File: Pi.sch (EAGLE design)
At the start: 9 parts, among them X1 RASPI_GPIO_B+#_BOX, X2 HDD, 5V 700mA

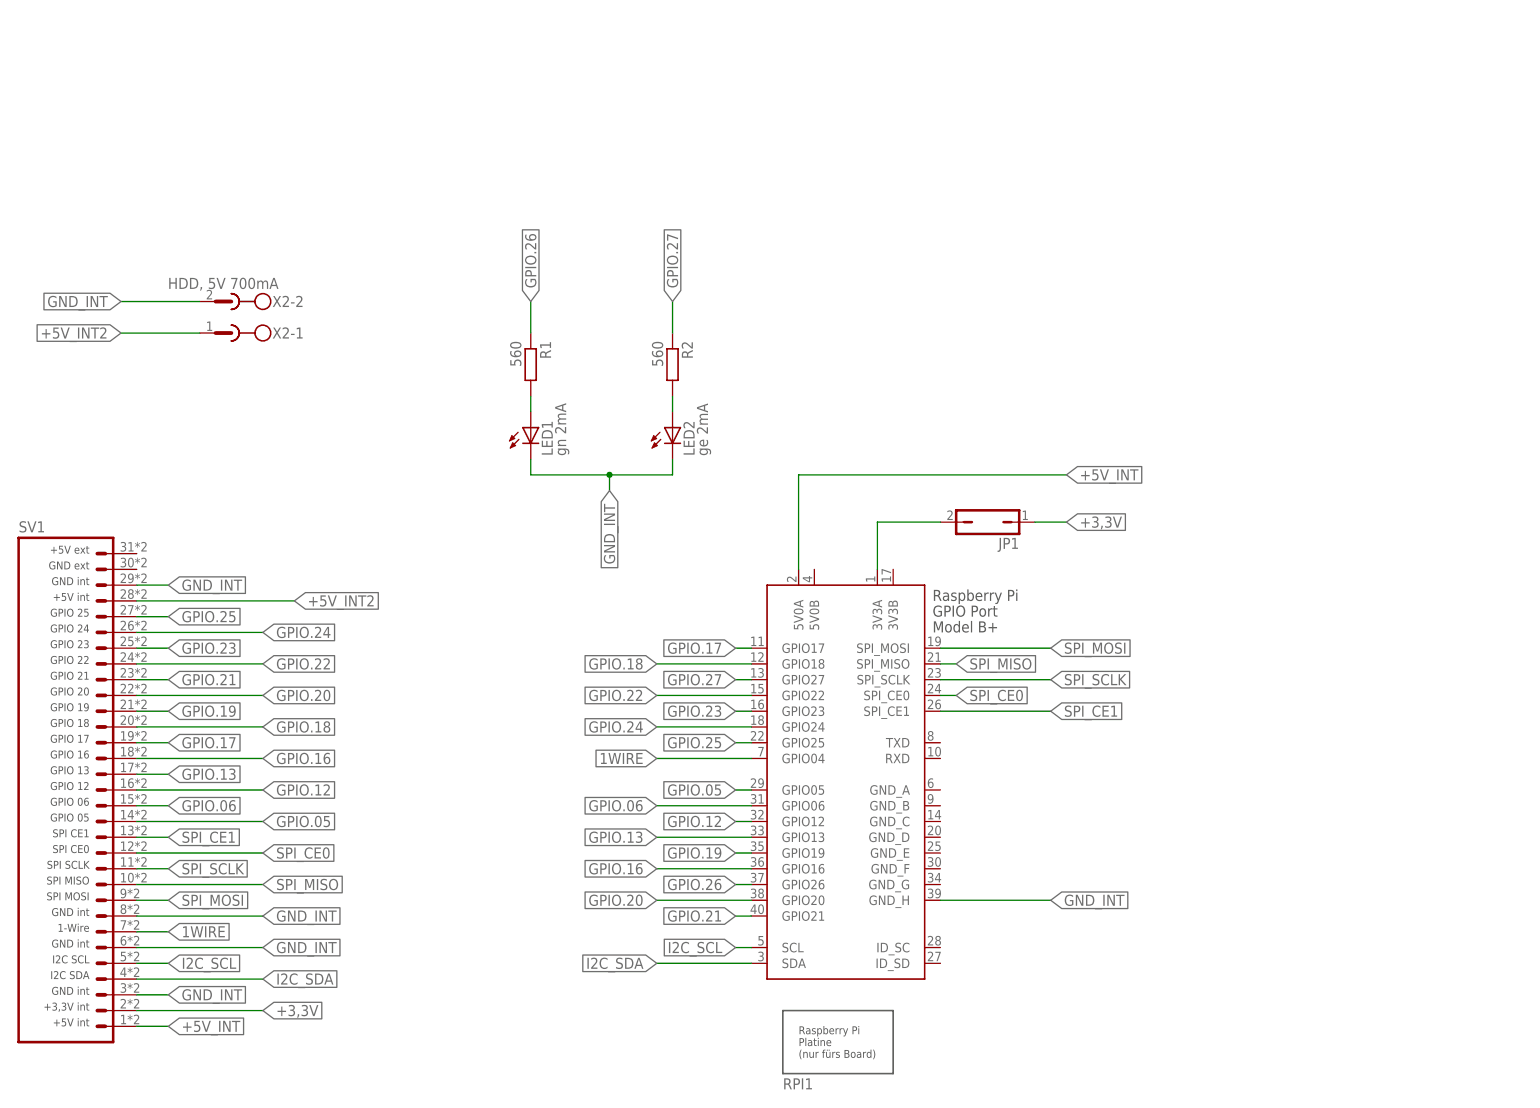
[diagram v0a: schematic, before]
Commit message: Pi und Stromversorgung Rev. 2019
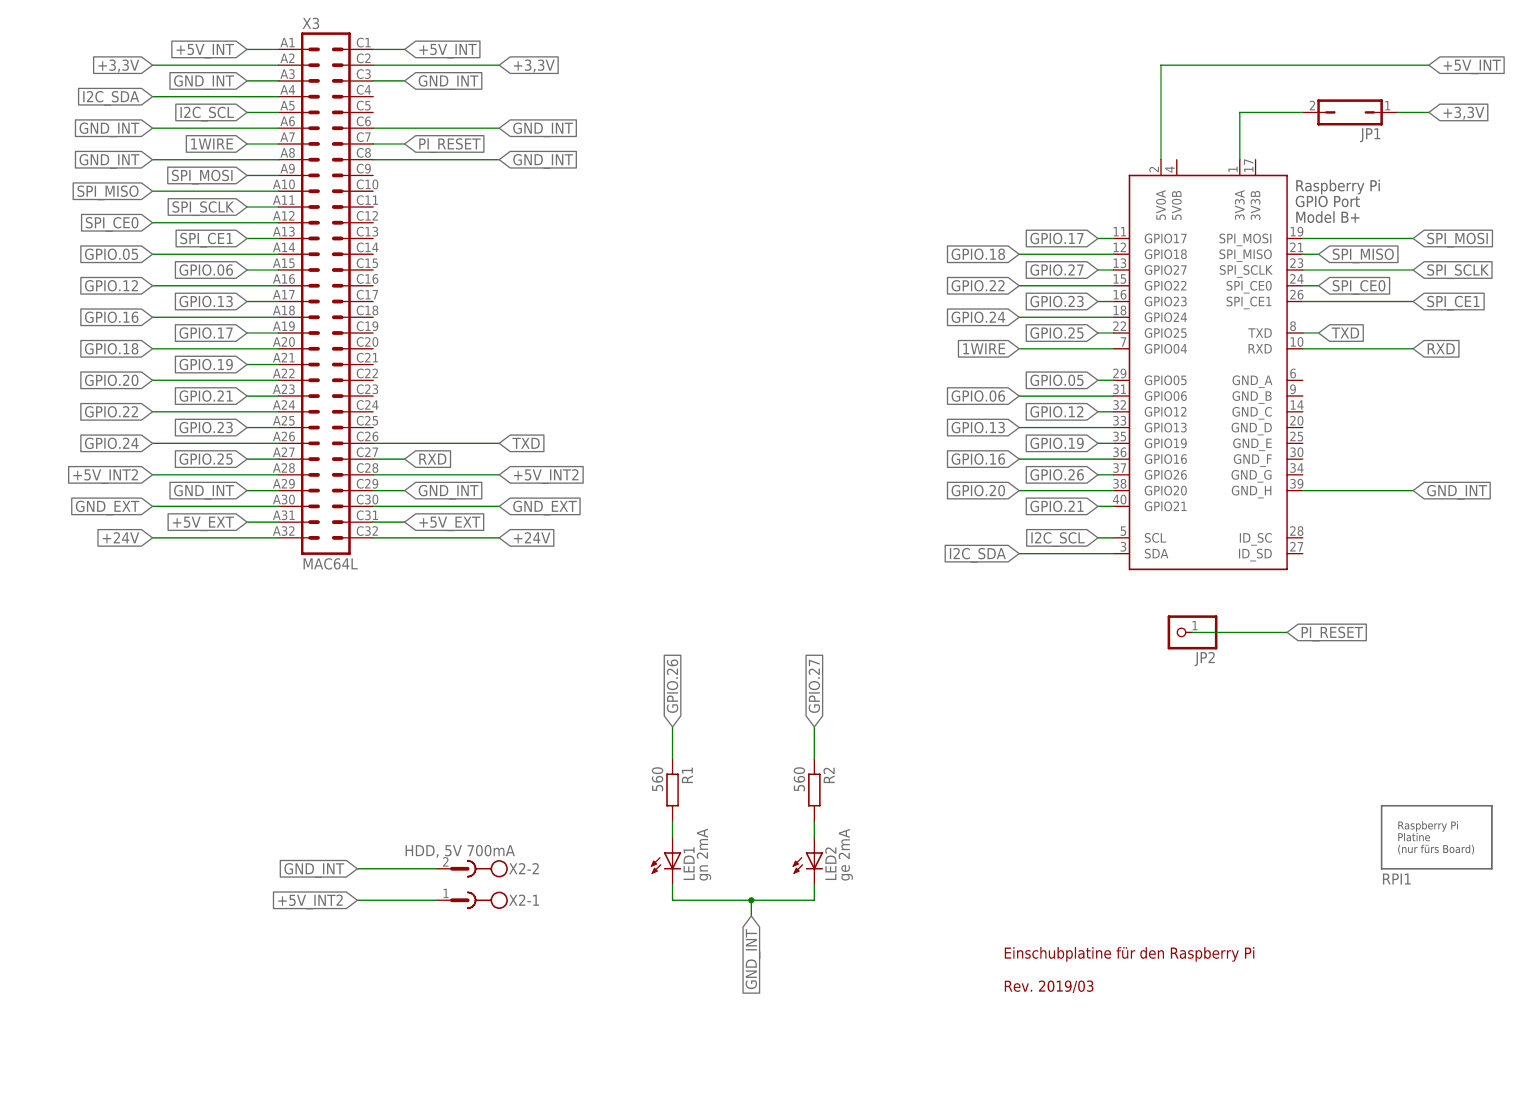
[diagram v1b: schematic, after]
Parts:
- removed SV1: PLATINENVERBINDER-31SMD, homepi:PLATINENVERBINDER-31SMD
- added JP2: (no value), pinhead:PINHD-1X1
- added X3: MAC64L, con-vg:MAC64L
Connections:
- new net +24V: X3.A32, X3.C32
- new net +5V_EXT: X3.A31, X3.C31
- new net GND_EXT: X3.A30, X3.C30
- new net PI_RESET: JP2.1, X3.C7
- new net RXD: X1.RXD, X3.C27
- new net TXD: X1.TXD, X3.C26
- net +3,3V: now also X3.A2, X3.C2; no longer SV1.2
- net +5V_INT: now also X3.A1, X3.C1; no longer SV1.1
- net +5V_INT2: now also X3.A28, X3.C28; no longer SV1.28
- net 1WIRE: now also X3.A7; no longer SV1.7
- net GND_INT: now also X3.A29, X3.A3, X3.A6, X3.A8, X3.C29, X3.C3, X3.C6, X3.C8; no longer SV1.29, SV1.3, SV1.6, SV1.8
- net GPIO.05: now also X3.A14; no longer SV1.14
- net GPIO.06: now also X3.A15; no longer SV1.15
- net GPIO.12: now also X3.A16; no longer SV1.16
- net GPIO.13: now also X3.A17; no longer SV1.17
- net GPIO.16: now also X3.A18; no longer SV1.18
- net GPIO.17: now also X3.A19; no longer SV1.19
- net GPIO.18: now also X3.A20; no longer SV1.20
- net GPIO.19: now also X3.A21; no longer SV1.21
- net GPIO.20: now also X3.A22; no longer SV1.22
- net GPIO.21: now also X3.A23; no longer SV1.23
- net GPIO.22: now also X3.A24; no longer SV1.24
- net GPIO.23: now also X3.A25; no longer SV1.25
- net GPIO.24: now also X3.A26; no longer SV1.26
- net GPIO.25: now also X3.A27; no longer SV1.27
- net I2C_SCL: now also X3.A5; no longer SV1.5
- net I2C_SDA: now also X3.A4; no longer SV1.4
- net SPI_CE0: now also X3.A12; no longer SV1.12
- net SPI_CE1: now also X3.A13; no longer SV1.13
- net SPI_MISO: now also X3.A10; no longer SV1.10
- net SPI_MOSI: now also X3.A9; no longer SV1.9
- net SPI_SCLK: now also X3.A11; no longer SV1.11
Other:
- note added: "Einschubplatine für den Raspberry Pi Rev. 2019/03"
- moved on the sheet: JP1, LED1, LED2, R1, R2, RPI1, X2-1, X2-2
